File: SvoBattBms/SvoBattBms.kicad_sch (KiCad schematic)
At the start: 1 part, among them U1 STM32F042K6Tx

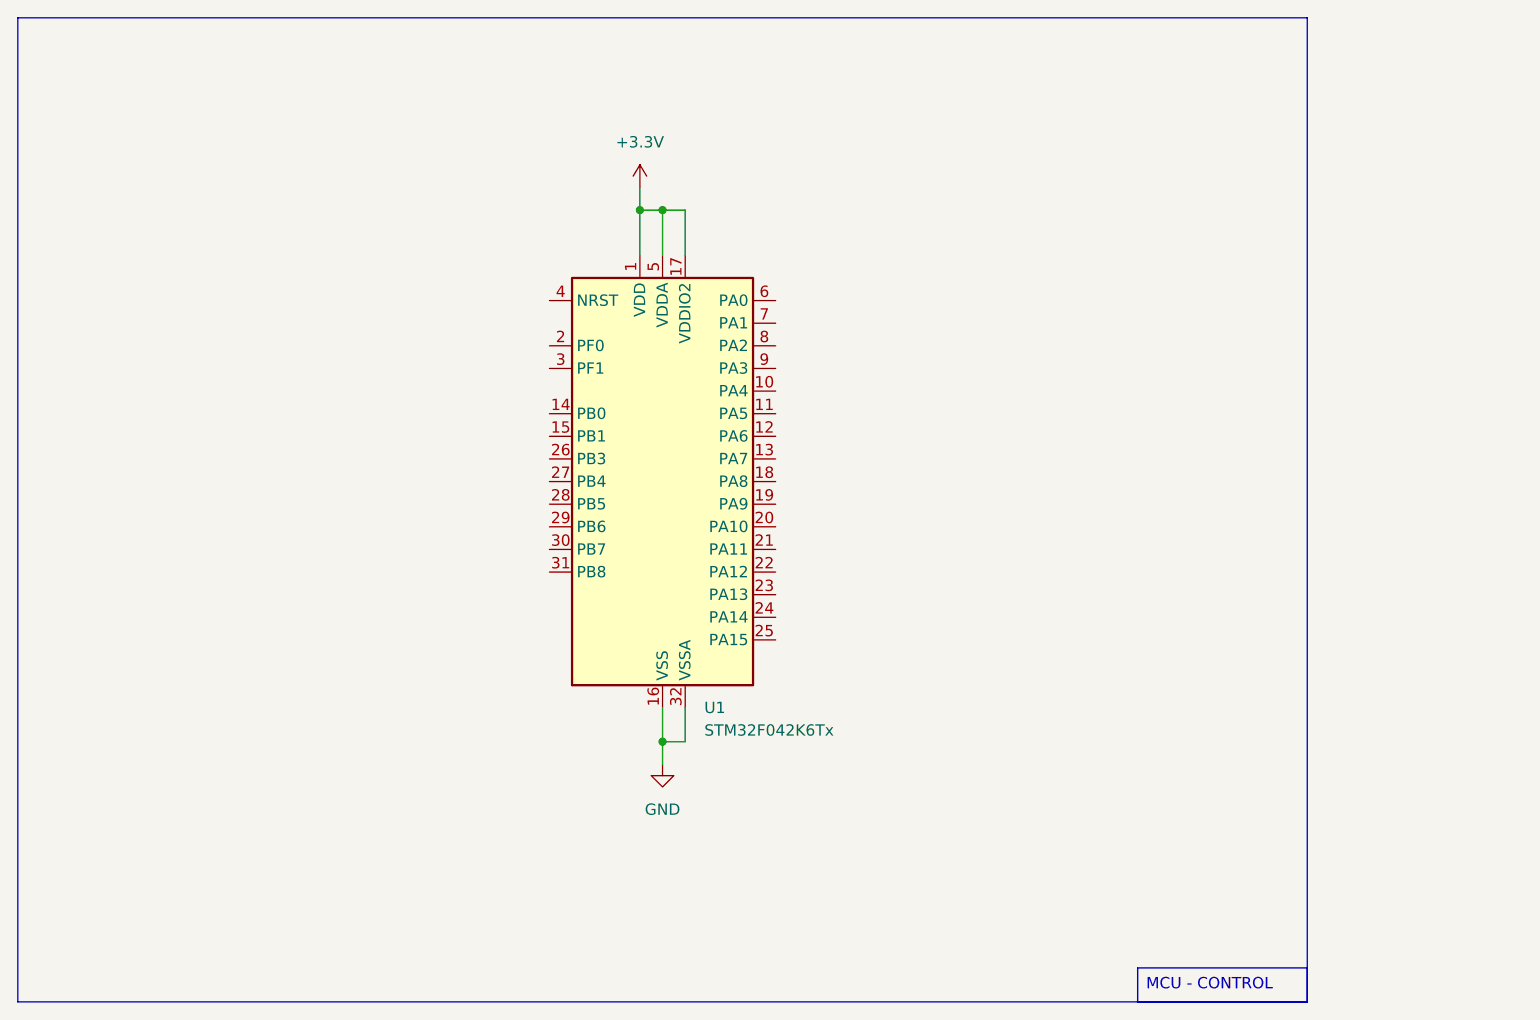
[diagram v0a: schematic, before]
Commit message: placa bms pronta
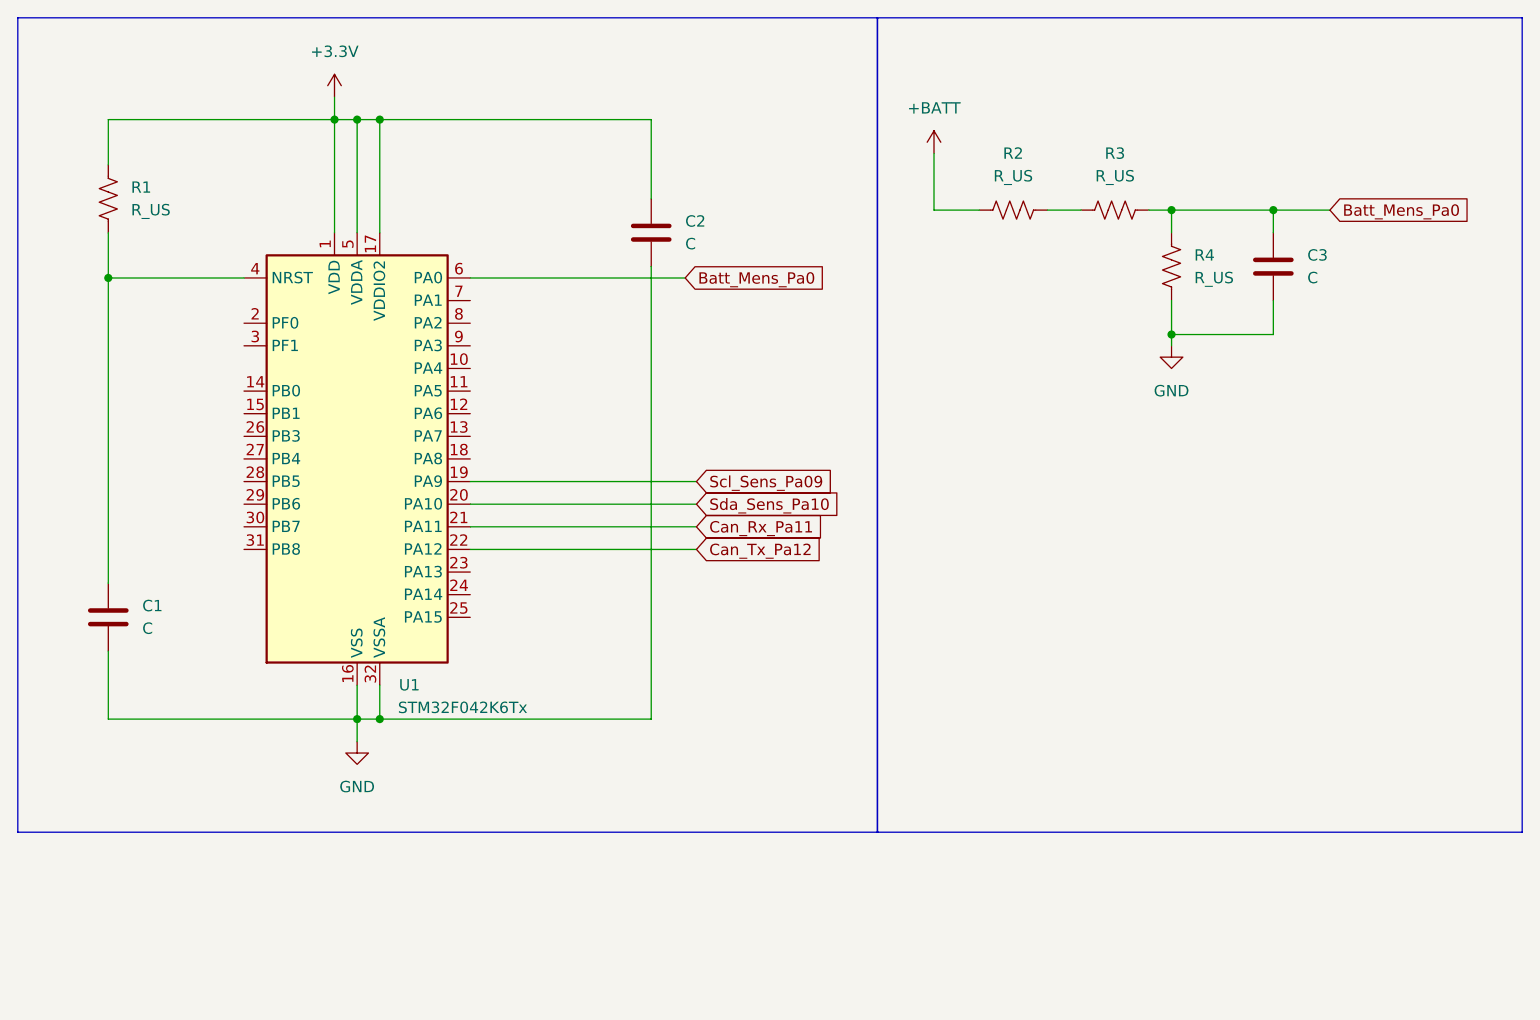
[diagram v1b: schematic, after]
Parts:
- added C1, C2, C3: C, symbol Device:C
- added R1, R2, R3, R4: R_US, symbol Device:R_US
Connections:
- net +3.3V: now also C2.1, R1.1
- net GND: now also C1.2, C2.2, C3.2, R4.2
- net Scl_Sens_Pa09: now reaches U1.19 (PA9)
- net Sda_Sens_Pa10: now reaches U1.20 (PA10)
- net Can_Rx_Pa11: now reaches U1.21 (PA11)
- net Can_Tx_Pa12: now reaches U1.22 (PA12)
- net at U1.4 (NRST): now also C1.1, R1.2
- net Batt_Mens_Pa0: now reaches U1.6 (PA0)
- net Batt_Mens_Pa0: now also C3.1, R3.2, R4.1
- new net: R2.2, R3.1
- new net +BATT: R2.1
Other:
- moved on the sheet: U1
